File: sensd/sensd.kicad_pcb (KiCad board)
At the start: 2 copper layers, 66 parts, among them J1 Conn_01x05, J10 Conn_01x05, J11 Conn_01x05, J12 Conn_02x05_Top_Bottom, J13 RJ45, J14 DE9_Plug, J15 Conn_01x02, J16 Conn_01x02, J17 Conn_01x02, J2 Conn_01x05, J3 Conn_01x05, J4 Conn_01x05, J5 Conn_01x05, J6 Conn_01x05, J7 Conn_01x05, J8 Conn_01x05, J9 Conn_01x05, Q1 Q_NMOS_GSD, Q10 Q_NMOS_GSD, Q11 Q_NMOS_GSD, Q12 Q_NMOS_GSD, Q13 Q_NMOS_GSD, Q2 Q_NMOS_GSD, Q3 Q_NMOS_GSD, Q4 Q_NMOS_GSD, Q5 Q_NMOS_GSD, Q6 Q_NMOS_GSD, Q7 Q_NMOS_GSD, Q8 Q_NMOS_GSD, Q9 Q_NMOS_GSD, SW1 RotaryEncoder_Switch, U1 Teensy4.1, U2 MAX3232, U3 XL1509-5.0

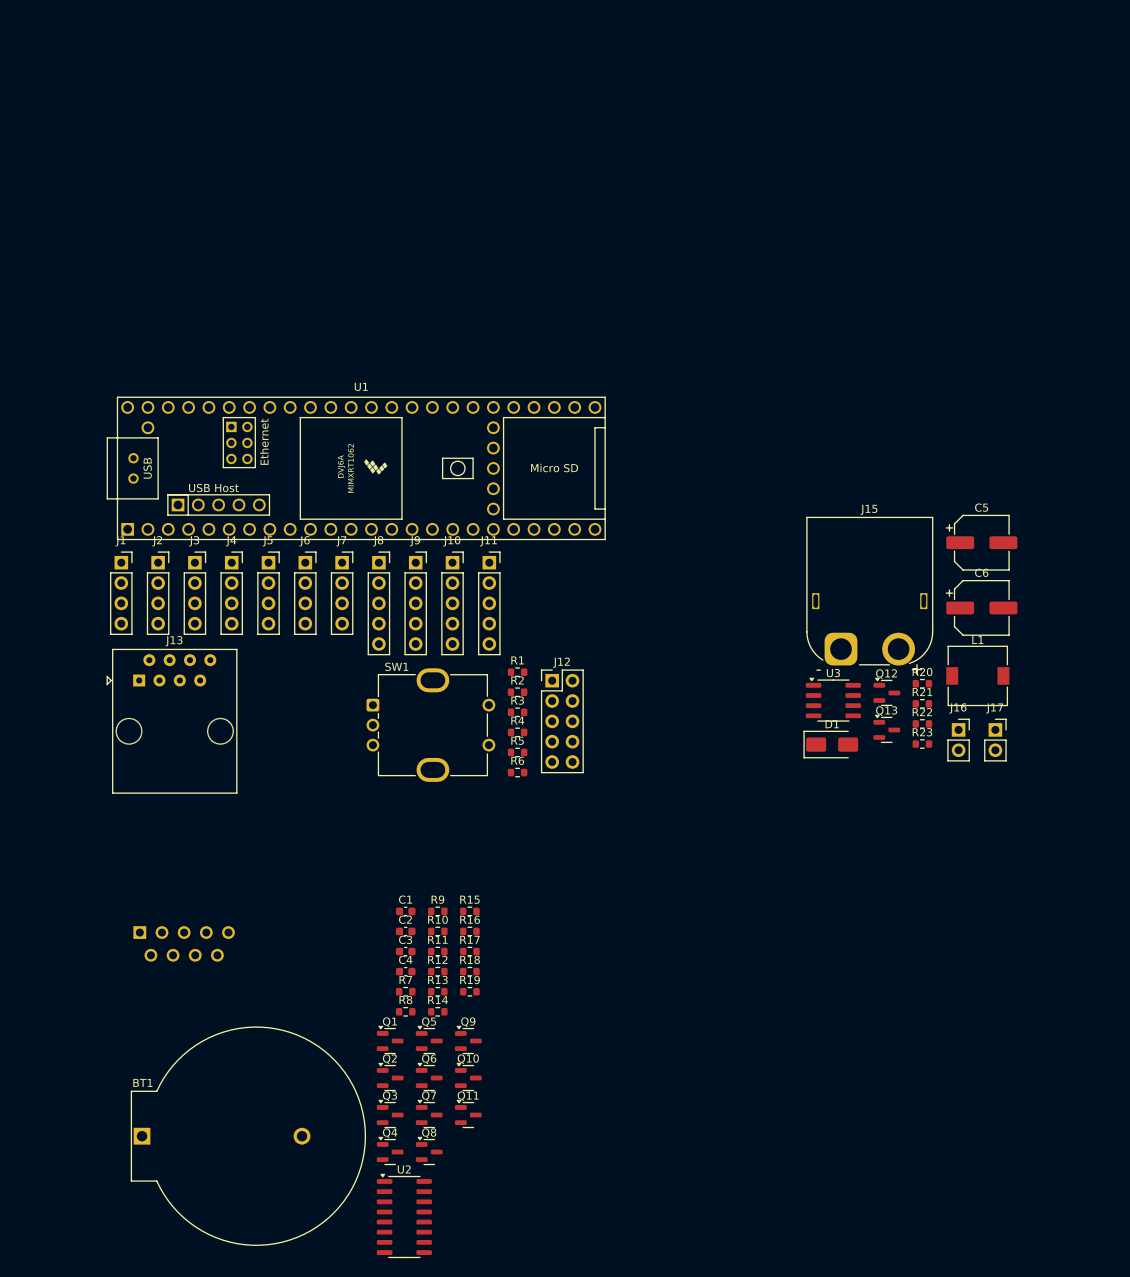
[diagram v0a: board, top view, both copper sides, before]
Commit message: board completed
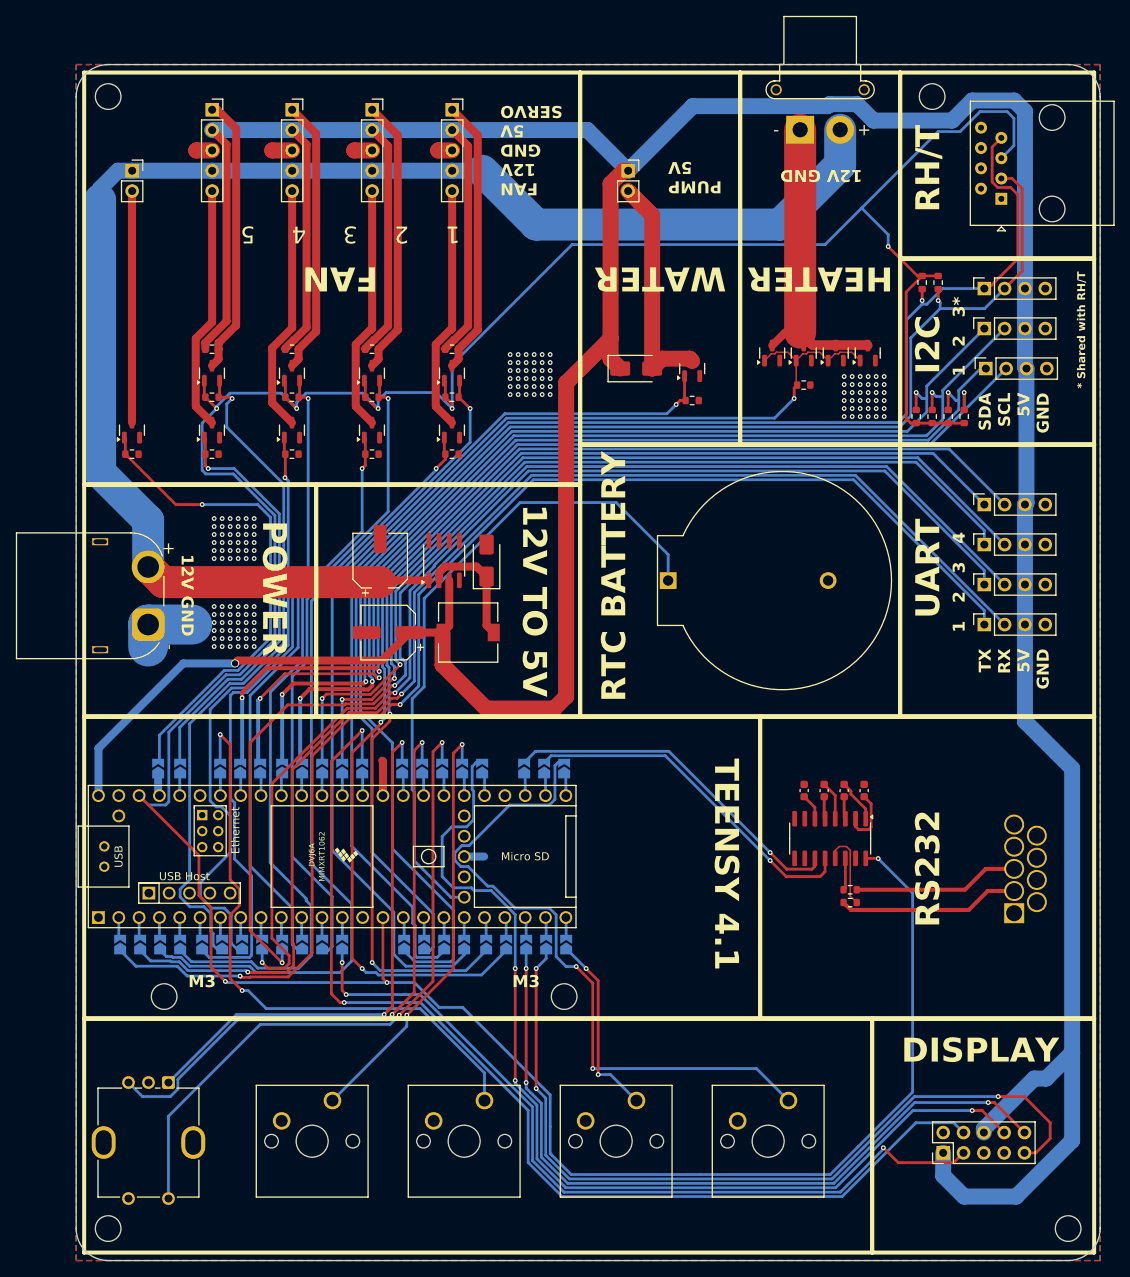
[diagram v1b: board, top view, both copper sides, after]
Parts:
- added D2: D, Diode_SMD:D_SMA, F.Cu at (99.0, 82.0)
- added J18: Conn_02x05_Top_Bottom, Connector_PinHeader_2.54mm:PinHeader_2x05_P2.54mm_Vertical, F.Cu at (137.4, 180.0)
- added JP10: SolderJumper_2_Open, Jumper:SolderJumper-2_P1.3mm_Open_TrianglePad1.0x1.5mm, B.Cu at (54.8, 154.0)
- added JP11: SolderJumper_2_Open, Jumper:SolderJumper-2_P1.3mm_Open_TrianglePad1.0x1.5mm, B.Cu at (57.2, 154.0)
- added JP12: SolderJumper_2_Open, Jumper:SolderJumper-2_P1.3mm_Open_TrianglePad1.0x1.5mm, B.Cu at (59.8, 154.0)
- added JP13: SolderJumper_2_Open, Jumper:SolderJumper-2_P1.3mm_Open_TrianglePad1.0x1.5mm, B.Cu at (62.2, 154.0)
- added JP15: SolderJumper_2_Open, Jumper:SolderJumper-2_P1.3mm_Open_TrianglePad1.0x1.5mm, B.Cu at (70.0, 154.0)
- added JP16: SolderJumper_2_Open, Jumper:SolderJumper-2_P1.3mm_Open_TrianglePad1.0x1.5mm, B.Cu at (72.5, 154.0)
- added JP17: SolderJumper_2_Open, Jumper:SolderJumper-2_P1.3mm_Open_TrianglePad1.0x1.5mm, B.Cu at (75.0, 154.0)
- added JP18: SolderJumper_2_Open, Jumper:SolderJumper-2_P1.3mm_Open_TrianglePad1.0x1.5mm, B.Cu at (77.5, 154.0)
- added JP19: SolderJumper_2_Open, Jumper:SolderJumper-2_P1.3mm_Open_TrianglePad1.0x1.5mm, B.Cu at (80.2, 154.0)
- added JP2: SolderJumper_2_Open, Jumper:SolderJumper-2_P1.3mm_Open_TrianglePad1.0x1.5mm, B.Cu at (34.5, 154.0)
- added JP20: SolderJumper_2_Open, Jumper:SolderJumper-2_P1.3mm_Open_TrianglePad1.0x1.5mm, B.Cu at (82.8, 154.0)
- added JP21: SolderJumper_2_Open, Jumper:SolderJumper-2_P1.3mm_Open_TrianglePad1.0x1.5mm, B.Cu at (85.2, 154.0)
- added JP22: SolderJumper_2_Open, Jumper:SolderJumper-2_P1.3mm_Open_TrianglePad1.0x1.5mm, B.Cu at (87.8, 154.0)
- added JP23: SolderJumper_2_Open, Jumper:SolderJumper-2_P1.3mm_Open_TrianglePad1.0x1.5mm, B.Cu at (90.2, 154.0)
- added JP27: SolderJumper_2_Open, Jumper:SolderJumper-2_P1.3mm_Open_TrianglePad1.0x1.5mm, B.Cu at (39.2, 132.0)
- added JP28: SolderJumper_2_Open, Jumper:SolderJumper-2_P1.3mm_Open_TrianglePad1.0x1.5mm, B.Cu at (42.0, 132.0)
- added JP29: SolderJumper_2_Open, Jumper:SolderJumper-2_P1.3mm_Open_TrianglePad1.0x1.5mm, B.Cu at (47.0, 132.0)
- added JP3: SolderJumper_2_Open, Jumper:SolderJumper-2_P1.3mm_Open_TrianglePad1.0x1.5mm, B.Cu at (37.0, 154.0)
- added JP30: SolderJumper_2_Open, Jumper:SolderJumper-2_P1.3mm_Open_TrianglePad1.0x1.5mm, B.Cu at (49.5, 132.0)
- added JP31: SolderJumper_2_Open, Jumper:SolderJumper-2_P1.3mm_Open_TrianglePad1.0x1.5mm, B.Cu at (52.0, 132.0)
- added JP32: SolderJumper_2_Open, Jumper:SolderJumper-2_P1.3mm_Open_TrianglePad1.0x1.5mm, B.Cu at (54.8, 132.0)
- added JP33: SolderJumper_2_Open, Jumper:SolderJumper-2_P1.3mm_Open_TrianglePad1.0x1.5mm, B.Cu at (57.2, 132.0)
- added JP34: SolderJumper_2_Open, Jumper:SolderJumper-2_P1.3mm_Open_TrianglePad1.0x1.5mm, B.Cu at (59.8, 132.0)
- added JP35: SolderJumper_2_Open, Jumper:SolderJumper-2_P1.3mm_Open_TrianglePad1.0x1.5mm, B.Cu at (62.2, 132.0)
- added JP36: SolderJumper_2_Open, Jumper:SolderJumper-2_P1.3mm_Open_TrianglePad1.0x1.5mm, B.Cu at (64.8, 132.0)
- added JP38: SolderJumper_2_Open, Jumper:SolderJumper-2_P1.3mm_Open_TrianglePad1.0x1.5mm, B.Cu at (69.8, 132.0)
- added JP39: SolderJumper_2_Open, Jumper:SolderJumper-2_P1.3mm_Open_TrianglePad1.0x1.5mm, B.Cu at (72.2, 132.0)
- added JP4: SolderJumper_2_Open, Jumper:SolderJumper-2_P1.3mm_Open_TrianglePad1.0x1.5mm, B.Cu at (39.5, 154.0)
- added JP40: SolderJumper_2_Open, Jumper:SolderJumper-2_P1.3mm_Open_TrianglePad1.0x1.5mm, B.Cu at (74.8, 132.0)
- added JP41: SolderJumper_2_Open, Jumper:SolderJumper-2_P1.3mm_Open_TrianglePad1.0x1.5mm, B.Cu at (77.2, 132.0)
- added JP42: SolderJumper_2_Open, Jumper:SolderJumper-2_P1.3mm_Open_TrianglePad1.0x1.5mm, B.Cu at (79.8, 132.0)
- added JP43: SolderJumper_2_Open, Jumper:SolderJumper-2_P1.3mm_Open_TrianglePad1.0x1.5mm, B.Cu at (85.0, 132.0)
- added JP44: SolderJumper_2_Open, Jumper:SolderJumper-2_P1.3mm_Open_TrianglePad1.0x1.5mm, B.Cu at (87.5, 132.0)
- added JP45: SolderJumper_2_Open, Jumper:SolderJumper-2_P1.3mm_Open_TrianglePad1.0x1.5mm, B.Cu at (90.0, 132.0)
- added JP5: SolderJumper_2_Open, Jumper:SolderJumper-2_P1.3mm_Open_TrianglePad1.0x1.5mm, B.Cu at (42.0, 154.0)
- added JP6: SolderJumper_2_Open, Jumper:SolderJumper-2_P1.3mm_Open_TrianglePad1.0x1.5mm, B.Cu at (44.8, 154.0)
- added JP7: SolderJumper_2_Open, Jumper:SolderJumper-2_P1.3mm_Open_TrianglePad1.0x1.5mm, B.Cu at (47.2, 154.0)
- added JP8: SolderJumper_2_Open, Jumper:SolderJumper-2_P1.3mm_Open_TrianglePad1.0x1.5mm, B.Cu at (49.8, 154.0)
- added JP9: SolderJumper_2_Open, Jumper:SolderJumper-2_P1.3mm_Open_TrianglePad1.0x1.5mm, B.Cu at (52.2, 154.0)
- added Q14: Q_NMOS_GSD, Package_TO_SOT_SMD:SOT-23, F.Cu at (116.0, 80.1)
- added REF**: MountingHole_3.2mm_M3, MountingHole:MountingHole_3.2mm_M3, F.Cu at (40.0, 160.5)
- added REF**: MountingHole_3.2mm_M3, MountingHole:MountingHole_3.2mm_M3, F.Cu at (90.0, 160.5)
- added REF**: MountingHole_3.2mm_M3, MountingHole:MountingHole_3.2mm_M3, F.Cu at (153.0, 189.5)
- added REF**: MountingHole_3.2mm_M3, MountingHole:MountingHole_3.2mm_M3, F.Cu at (33.0, 189.5)
- added REF**: MountingHole_3.2mm_M3, MountingHole:MountingHole_3.2mm_M3, F.Cu at (136.0, 48.0)
- added REF**: MountingHole_3.2mm_M3, MountingHole:MountingHole_3.2mm_M3, F.Cu at (33.0, 48.0)
- added SW2: SW_Push, Button_Switch_Keyboard:SW_Cherry_MX_1.00u_PCB, F.Cu at (61.0, 173.5)
- added SW3: SW_Push, Button_Switch_Keyboard:SW_Cherry_MX_1.00u_PCB, F.Cu at (80.0, 173.5)
- added SW4: SW_Push, Button_Switch_Keyboard:SW_Cherry_MX_1.00u_PCB, F.Cu at (99.0, 173.5)
- added SW5: SW_Push, Button_Switch_Keyboard:SW_Cherry_MX_1.00u_PCB, F.Cu at (118.0, 173.5)
- C1, C2, C3, C4: value C -> 100nF
- C5, C6: value C_Polarized -> 220uF
- J12: value Conn_02x05_Top_Bottom -> Conn_01x02; footprint Connector_PinHeader_2.54mm:PinHeader_2x05_P2.54mm_Vertical -> Connector_AMASS:AMASS_XT30PW-F_1x02_P2.50mm_Horizontal
- L1: value L -> 33uH
- R20, R21: value R -> 0
- moved J17 128.6 mm to (36.0, 57.3)
- moved J13 123.4 mm to (144.7, 60.8), turned to 90 degrees
- moved J14 109.3 mm to (146.2, 150.1), turned to -90 degrees
- moved J1 108.2 mm to (142.5, 114.0), turned to 90 degrees
- moved Q11 107.5 mm to (128.0, 80.1), turned to 90 degrees
- moved R23 105.2 mm to (36.0, 92.7), turned to 180 degrees
- moved J2 103.3 mm to (142.5, 109.0), turned to 90 degrees
- moved Q10 101.6 mm to (124.0, 80.1), turned to 90 degrees
- moved Q13 101.5 mm to (36.0, 89.7), turned to 90 degrees
- moved Q4 99.9 mm to (46.0, 82.6), turned to 90 degrees
- moved J3 98.7 mm to (142.5, 104.0), turned to 90 degrees
- moved Q9 95.7 mm to (120.0, 80.1), turned to 90 degrees
- moved BT1 95.6 mm to (103.0, 108.5)
- moved J4 94.4 mm to (142.5, 99.0), turned to 90 degrees
- moved Q8 94.2 mm to (46.0, 89.7), turned to 90 degrees
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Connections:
- BT1 pad 2: Net-(BT1--) -> GND
- J12 pad 2: Net-(J12-Pin_1) -> +12V
- J15 pad 1: unconnected-(J15-Pin_1-Pad1) -> GND
- J15 pad 2: unconnected-(J15-Pin_2-Pad2) -> +12V
- J16 pad 1: unconnected-(J16-Pin_1-Pad1) -> +5V
- R5 pad 1: unconnected-(R5-Pad1) -> +3V3
- U1 pad 10: unconnected-(U1-8_TX2_IN1-Pad10) -> Net-(JP10-B)
- U1 pad 11: unconnected-(U1-9_OUT1C-Pad11) -> Net-(JP11-B)
- U1 pad 12: unconnected-(U1-10_CS_MQSR-Pad12) -> Net-(JP12-B)
- U1 pad 13: unconnected-(U1-11_MOSI_CTX1-Pad13) -> Net-(JP13-B)
- U1 pad 16: unconnected-(U1-24_A10_TX6_SCL2-Pad16) -> Net-(JP15-B)
- U1 pad 17: unconnected-(U1-25_A11_RX6_SDA2-Pad17) -> Net-(JP16-B)
- U1 pad 18: unconnected-(U1-26_A12_MOSI1-Pad18) -> Net-(JP17-B)
- U1 pad 19: unconnected-(U1-27_A13_SCK1-Pad19) -> Net-(JP18-B)
- U1 pad 2: unconnected-(U1-0_RX1_CRX2_CS1-Pad2) -> Net-(JP2-B)
- U1 pad 20: unconnected-(U1-28_RX7-Pad20) -> Net-(JP19-B)
- U1 pad 21: unconnected-(U1-29_TX7-Pad21) -> Net-(JP20-B)
- U1 pad 22: unconnected-(U1-30_CRX3-Pad22) -> Net-(JP21-B)
- U1 pad 23: unconnected-(U1-31_CTX3-Pad23) -> Net-(JP22-B)
- U1 pad 24: unconnected-(U1-32_OUT1B-Pad24) -> Net-(JP23-B)
- U1 pad 25: unconnected-(U1-33_MCLK2-Pad25) -> Net-(JP45-A)
- U1 pad 26: unconnected-(U1-34_RX8-Pad26) -> Net-(JP44-A)
- U1 pad 27: unconnected-(U1-35_TX8-Pad27) -> Net-(JP43-A)
- U1 pad 29: unconnected-(U1-37_CS-Pad29) -> Net-(JP42-A)
- U1 pad 3: unconnected-(U1-1_TX1_CTX2_MISO1-Pad3) -> Net-(JP3-B)
- U1 pad 30: unconnected-(U1-38_CS1_IN1-Pad30) -> Net-(JP41-A)
- U1 pad 31: unconnected-(U1-39_MISO1_OUT1A-Pad31) -> Net-(JP40-A)
- U1 pad 32: unconnected-(U1-40_A16-Pad32) -> Net-(JP39-A)
- U1 pad 33: unconnected-(U1-41_A17-Pad33) -> Net-(JP38-A)
- U1 pad 35: unconnected-(U1-13_SCK_LED-Pad35) -> Net-(JP36-A)
- U1 pad 36: unconnected-(U1-14_A0_TX3_SPDIF_OUT-Pad36) -> Net-(JP35-A)
- U1 pad 37: unconnected-(U1-15_A1_RX3_SPDIF_IN-Pad37) -> Net-(JP34-A)
- U1 pad 38: unconnected-(U1-16_A2_RX4_SCL1-Pad38) -> Net-(JP33-A)
- U1 pad 39: unconnected-(U1-17_A3_TX4_SDA1-Pad39) -> Net-(JP32-A)
- U1 pad 4: unconnected-(U1-2_OUT2-Pad4) -> Net-(JP4-B)
- U1 pad 40: unconnected-(U1-18_A4_SDA-Pad40) -> Net-(JP31-A)
- U1 pad 41: unconnected-(U1-19_A5_SCL-Pad41) -> Net-(JP30-A)
- U1 pad 42: unconnected-(U1-20_A6_TX5_LRCLK1-Pad42) -> Net-(JP29-A)
- U1 pad 44: unconnected-(U1-22_A8_CTX1-Pad44) -> Net-(JP28-A)
- U1 pad 45: unconnected-(U1-23_A9_CRX1_MCLK1-Pad45) -> Net-(JP27-A)
- U1 pad 5: unconnected-(U1-3_LRCLK2-Pad5) -> Net-(JP5-B)
- U1 pad 52: Net-(BT1--) -> GND
- U1 pad 6: unconnected-(U1-4_BCLK2-Pad6) -> Net-(JP6-B)
- U1 pad 7: unconnected-(U1-5_IN2-Pad7) -> Net-(JP7-B)
- U1 pad 8: unconnected-(U1-6_OUT1D-Pad8) -> Net-(JP8-B)
- U1 pad 9: unconnected-(U1-7_RX2_OUT1A-Pad9) -> Net-(JP9-B)
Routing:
- net +5V: track 0.00 -> 554.3 mm, vias 0 -> 1
- net +3V3: track 0.00 -> 426.6 mm, vias 0 -> 8
- net +12V: track 0.00 -> 189.4 mm
- net /SCL3: track 0.00 -> 179.7 mm, vias 0 -> 1
- net /SDA3: track 0.00 -> 177.6 mm, vias 0 -> 1
- net /RX1: track 0.00 -> 164.9 mm, vias 0 -> 2
- net /TX1: track 0.00 -> 163.7 mm, vias 0 -> 2
- net /TX4: track 0.00 -> 157.5 mm, vias 0 -> 2
- net /TX2: track 0.00 -> 152.5 mm, vias 0 -> 2
- net /RX4: track 0.00 -> 147.9 mm, vias 0 -> 2
- net /RX2: track 0.00 -> 147.4 mm, vias 0 -> 2
- net /HEATER: track 0.00 -> 139.0 mm, vias 0 -> 1
- net /SCK: track 0.00 -> 136.2 mm, vias 0 -> 2
- net /SCL1: track 0.00 -> 132.5 mm, vias 0 -> 3
- net /SDA1: track 0.00 -> 129.9 mm, vias 0 -> 3
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- added copper zone on B.Cu, net GND
- added copper zone on F.Cu, net GND
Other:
- board outline added: 128 x 149.5 mm
- board text added: "* Shared with RH/T"
- board text added: "1 2 3 4"
- board text added: "1 2 3 4 5"
- board text added: "1 2 3*"
- board text added: "12V GND"
- board text added: "12V TO 5V"
- board text added: "DISPLAY"
- board text added: "Environmental air chamber PCB V0.1 https://github.com/ReFil/Sensor-test/tree/main/sensd"
- board text added: "FAN"
- board text added: "FAN 12V GND 5V SERVO"
- board text added: "HEATER"
- board text added: "I2C"
- board text added: "M3"
- board text added: "POWER"
- board text added: "PUMP 5V"
- board text added: "RH/T"
- board text added: "RS232"
- board text added: "RTC BATTERY"
- board text added: "SDA SCL 5V GND"
- board text added: "TEENSY 4.1"
- board text added: "TX RX 5V GND"
- board text added: "UART"
- board text added: "WATER"
